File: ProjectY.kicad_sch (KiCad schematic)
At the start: 8 parts, among them J2 NRJ6HF, J3 9V, J4 NRJ6HF, J5 NRJ6HF, J6 AudioJack3, J7 AudioJack3, P1 USB_C

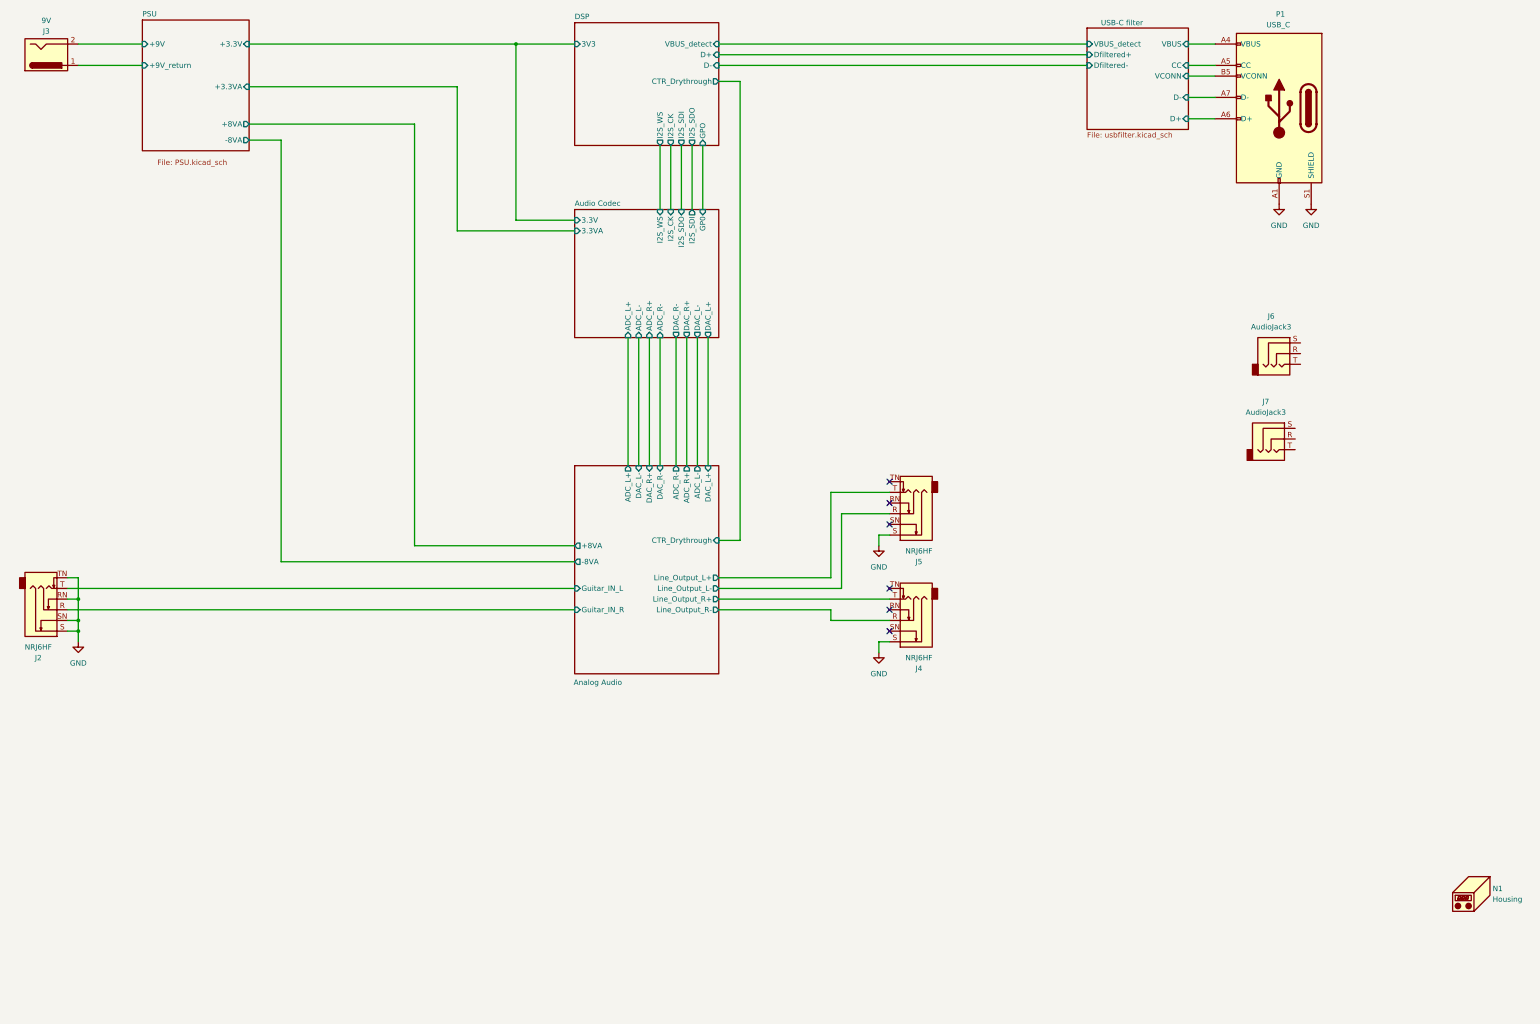
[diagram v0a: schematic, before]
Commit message: modified:   MCU.kicad_sch 	modified:   PSU.kicad_sch 	modified:   ProjectY.kicad_pro 	modified:   ProjectY.kicad_sch 	modified:   ad.kicad_sch 	modified:   audio.kicad_sch
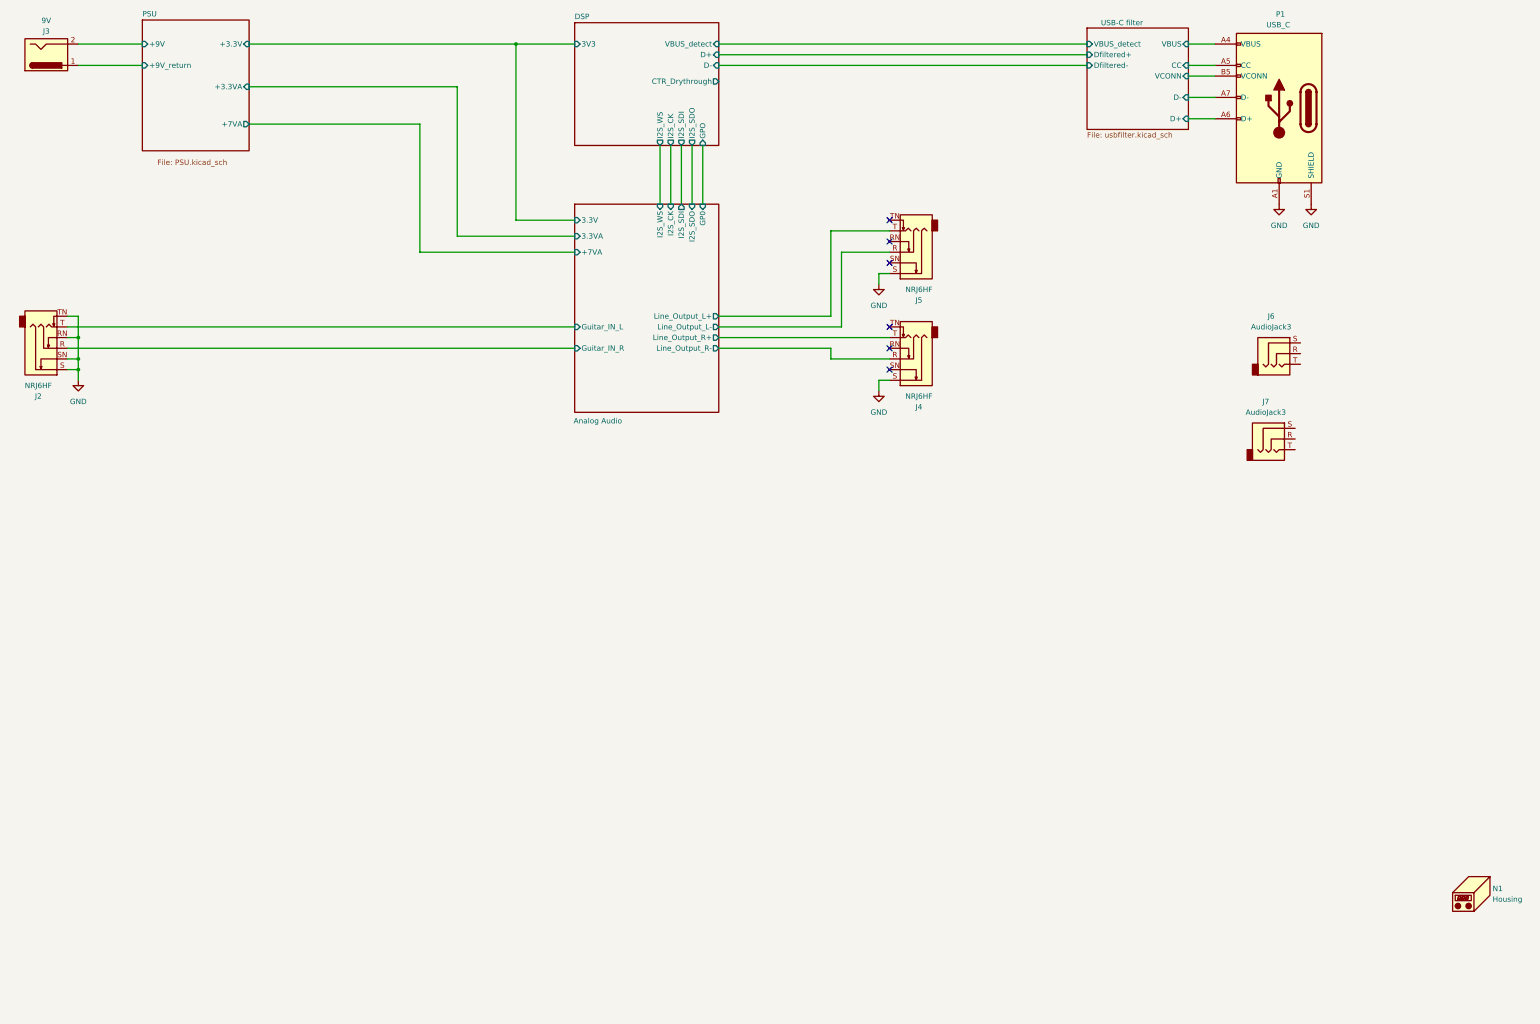
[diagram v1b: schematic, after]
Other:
- removed sheet Audio Codec
- sheet Analog Audio ports: added +7VA, 3.3V, 3.3VA, GP0, I2S_CK, I2S_SDI, I2S_SDO, I2S_WS; removed +8VA, -8VA, ADC_L+, ADC_L-, ADC_R+, ADC_R-, CTR_Drythrough, DAC_L+, DAC_L-, DAC_R+, DAC_R-
- sheet PSU ports: added +7VA; removed +8VA, -8VA
- moved on the sheet: J2, J4, J5

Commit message: modified:   MCU.kicad_sch 	modified:   PSU.kicad_sch 	modified:   ProjectY.kicad_pro 	modified:   ProjectY.kicad_sch 	modified:   audio.kicad_sch 	modified:   fp-info-cache 	new file:   spdif.kicad_sch 	modified:   usbfilter.kicad_sch
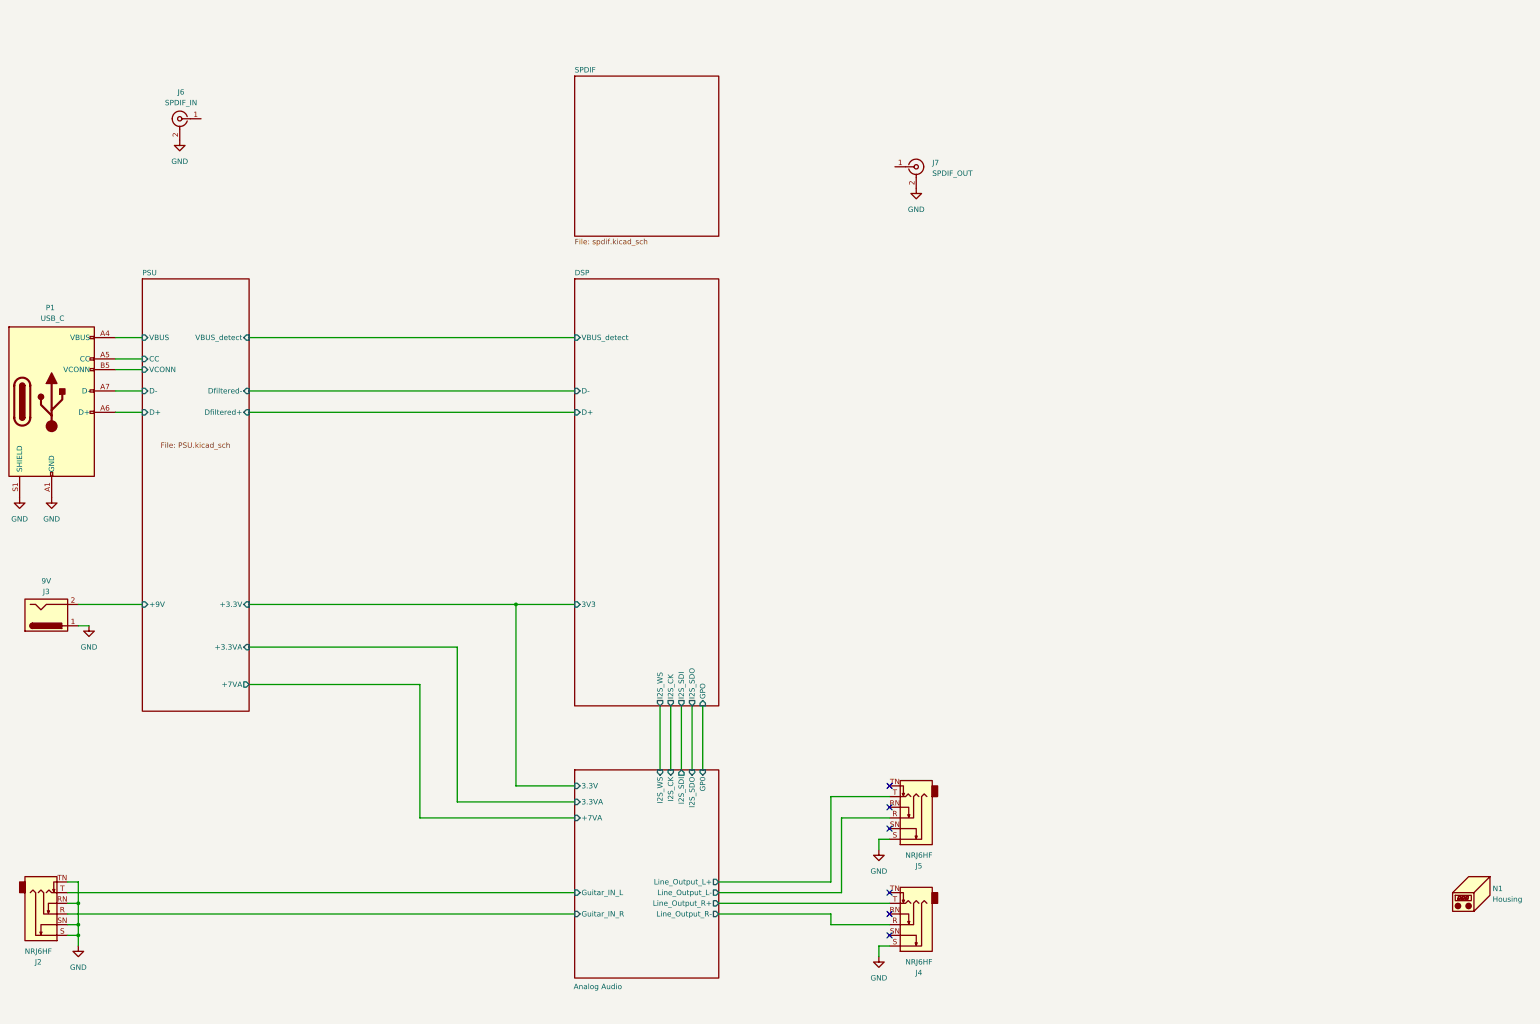
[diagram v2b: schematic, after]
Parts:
- removed J6, J7: AudioJack3, Connector_Audio:Jack_3.5mm_CUI_SJ-3523-SMT_Horizontal, symbol Connector_Audio:AudioJack3
- added J6: SPDIF_IN, symbol Connector:Conn_Coaxial
- added J7: SPDIF_OUT, symbol Connector:Conn_Coaxial
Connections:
- net PSU/+9V_return is gone; now on net GND: J3.1
- net GND: now also J6.2 (Ext), J7.2 (Ext)
- net USB-C filter/CC renamed PSU/CC
- net USB-C filter/D+ renamed PSU/D+
- net USB-C filter/D- renamed PSU/D-
- net USB-C filter/VBUS renamed PSU/VBUS
- net USB-C filter/VCONN renamed PSU/VCONN
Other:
- removed sheet USB-C filter
- added sheet SPDIF (spdif.kicad_sch)
- sheet DSP ports: added none; removed CTR_Drythrough
- sheet PSU ports: added CC, D+, D-, Dfiltered+, Dfiltered-, VBUS, VBUS_detect, VCONN; removed +9V_return
- moved on the sheet: J2, J3, J4, J5, P1

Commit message: asd
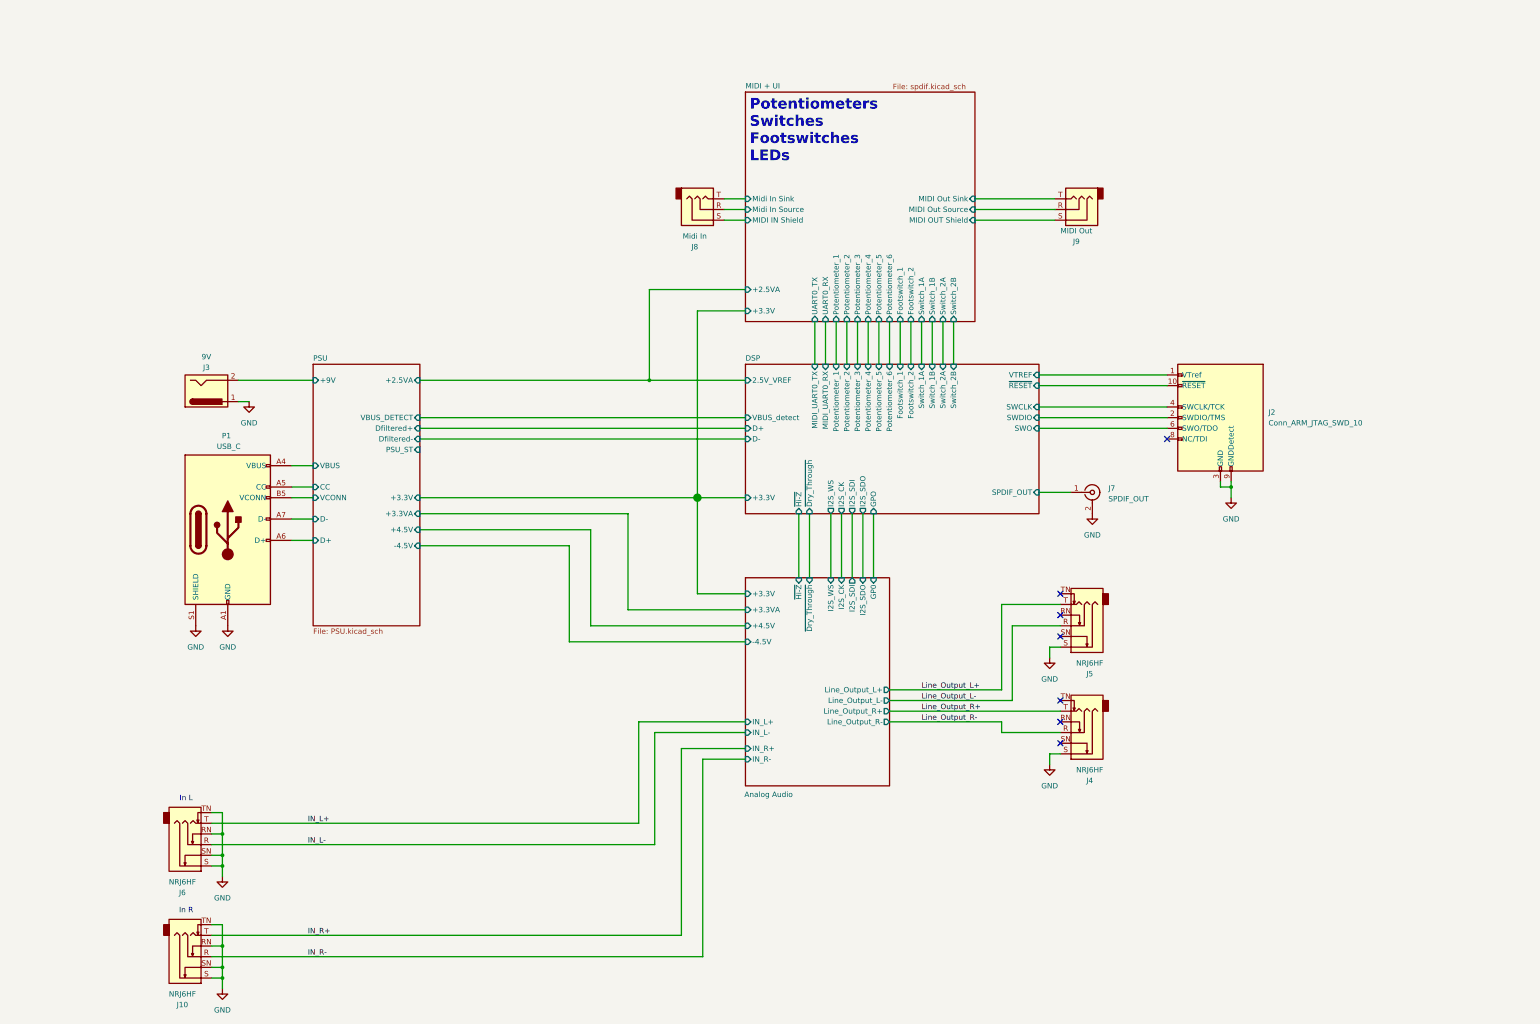
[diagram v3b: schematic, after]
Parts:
- removed J2: NRJ6HF, Connector_Audio:Jack_6.35mm_Neutrik_NRJ6HF_Horizontal, symbol Connector_Audio:NRJ6HF
- removed J6: SPDIF_IN, symbol Connector:Conn_Coaxial
- removed N1: Housing, Enclosures:Hammond_1590BB, symbol Mechanical:Housing
- added J10, J6: NRJ6HF, Connector_Audio:Jack_6.35mm_Neutrik_NRJ6HF_Horizontal, symbol Connector_Audio:NRJ6HF
- added J2: Conn_ARM_JTAG_SWD_10, symbol Connector:Conn_ARM_JTAG_SWD_10
- added J8: Midi In, Connector_Audio:Jack_3.5mm_Lumberg_1503_07_Horizontal, symbol Connector_Audio:AudioJack3
- added J9: MIDI Out, Connector_Audio:Jack_3.5mm_Lumberg_1503_07_Horizontal, symbol Connector_Audio:AudioJack3
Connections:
- net GND: now also J10.RN, J10.S, J10.SN, J10.TN, J2.3 (GND), J2.5 (GND), J2.9 (GNDDetect), J6.RN, J6.S, J6.SN, J6.TN
- net DSP/SPDIF_OUT: now reaches J7.1 (In)
- net Analog Audio/Line_Output_L+ renamed Line_Output_L+
- net Analog Audio/Line_Output_L- renamed Line_Output_L-
- net Analog Audio/Line_Output_R+ renamed Line_Output_R+
- net Analog Audio/Line_Output_R- renamed Line_Output_R-
- new net DSP/SWCLK: J2.4 (SWCLK/TCK)
- new net DSP/SWDIO: J2.2 (SWDIO/TMS)
- new net DSP/SWO: J2.6 (SWO/TDO)
- new net DSP/VTREF: J2.1 (VTref)
- new net DSP/~{RESET}: J2.10 (~{RESET})
- new net IN_L+: J6.T
- new net IN_L-: J6.R
- new net IN_R+: J10.T
- new net IN_R-: J10.R
- new net MIDI + UI/MIDI IN Shield: J8.S
- new net MIDI + UI/MIDI OUT Shield: J9.S
- new net MIDI + UI/MIDI Out Sink: J9.T
- new net MIDI + UI/MIDI Out Source: J9.R
- new net MIDI + UI/Midi In Sink: J8.T
- new net MIDI + UI/Midi In Source: J8.R
- no-connect marks 6 -> 7
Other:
- sheet SPDIF renamed MIDI + UI
- sheet Analog Audio ports: added +3.3V, +3.3VA, +4.5V, -4.5V, IN_L+, IN_L-, IN_R+, IN_R-, ~{Dry_Through}, ~{Hi-Z}; removed +7VA, 3.3V, 3.3VA, Guitar_IN_L, Guitar_IN_R
- sheet DSP ports: added +3.3V, 2.5V_VREF, Footswitch_1, Footswitch_2, MIDI_UART0_RX, MIDI_UART0_TX, Potentiometer_1, Potentiometer_2, Potentiometer_3, Potentiometer_4, Potentiometer_5, Potentiometer_6, SPDIF_OUT, SWCLK, SWDIO, SWO, Switch_1A, Switch_1B, Switch_2A, Switch_2B, VTREF, ~{Dry_Through}, ~{Hi-Z}, ~{RESET}; removed 3V3
- sheet MIDI + UI ports: added +2.5VA, +3.3V, Footswitch_1, Footswitch_2, MIDI IN Shield, MIDI OUT Shield, MIDI Out Sink, MIDI Out Source, Midi In Sink, Midi In Source, Potentiometer_1, Potentiometer_2, Potentiometer_3, Potentiometer_4, Potentiometer_5, Potentiometer_6, Switch_1A, Switch_1B, Switch_2A, Switch_2B, UART0_RX, UART0_TX; removed none
- sheet PSU ports: added +2.5VA, +4.5V, -4.5V, PSU_ST, VBUS_DETECT; removed +7VA, VBUS_detect
- note added: "In L"
- note added: "In R"
- note added: "Potentiometers Switches Footswitches LEDs"
- moved on the sheet: J3, J4, J5, J7, P1
